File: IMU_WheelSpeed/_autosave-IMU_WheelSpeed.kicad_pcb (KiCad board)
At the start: 2 copper layers, 23 parts, among them J1 Conn_01x06_Socket, J3 Conn_01x03_Socket, U1 PeripheralSOM, U2 LSM6DSL, U4 TPS71518__SC70

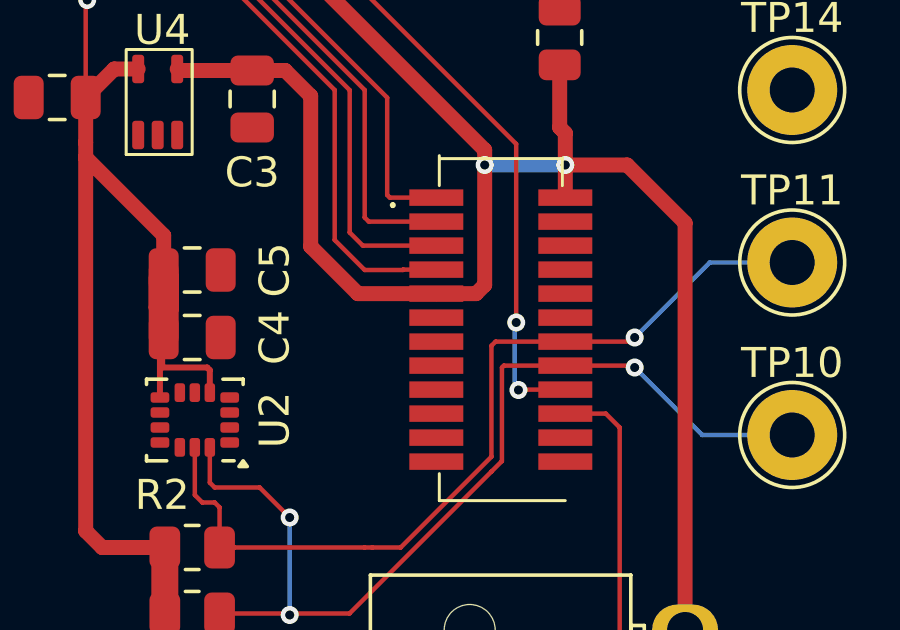
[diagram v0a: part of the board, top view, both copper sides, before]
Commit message: Check up
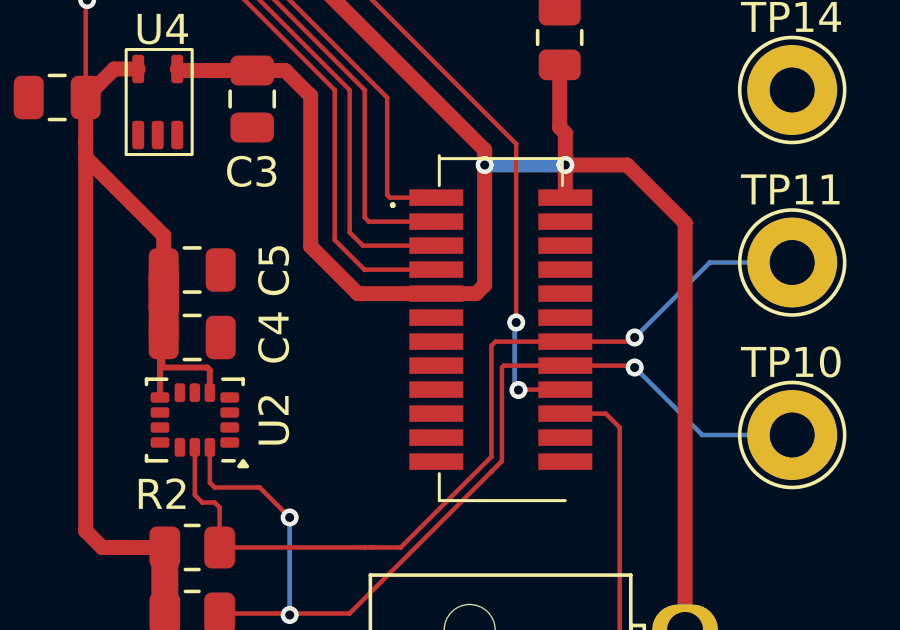
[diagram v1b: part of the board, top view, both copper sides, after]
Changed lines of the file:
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@@
+	)
+	(segment
+		(start 146.25 70.25)
+		(end 145.75 69.75)
+		(width 0.15)
+		(layer "F.Cu")
+		(net 2)
+	)
+	(segment
+		(start 161.13726 84.93726)
+		(end 158.68726 84.93726)
+		(width 0.15)
+		(layer "F.Cu")
+		(net 2)
+	)
+	(segment
+		(start 158.25 79.755025)
+		(end 148.744975 70.25)
+		(width 0.15)
+		(layer "F.Cu")
+		(net 2)
+	)
+	(segment
+		(start 145.75 69.75)
+		(end 145.75 61.93)
+		(width 0.15)
+		(layer "F.Cu")
+		(net 2)
 	)
 	(segment
 		(start 148.744975 70.25)
 		(end 146.25 70.25)
-		(width 0.15)
-		(layer "F.Cu")
-		(net 2)
-	)
-	(segment
-		(start 146.25 70.25)
-		(end 145.75 69.75)
-		(width 0.15)
-		(layer "F.Cu")
-		(net 2)
-	)
-	(segment
-		(start 145.75 69.75)
-		(end 145.75 61.93)
-		(width 0.15)
-		(layer "F.Cu")
-		(net 2)
-	)
-	(segment
-		(start 161.13726 84.93726)
-		(end 158.68726 84.93726)
-		(width 0.15)
-		(layer "F.Cu")
-		(net 2)
-	)
-	(segment
-		(start 158.25 79.755025)
-		(end 148.744975 70.25)
 		(width 0.15)
 		(layer "F.Cu")
@@
 	)
 	(segment
-		(start 163.87476 89.75)
-		(end 163.8875 89.73726)
-		(width 0.15)
-		(layer "F.Cu")
-		(net 5)
-	)
-	(segment
 		(start 163.8 81.55)
 		(end 155.75 73.5)
@@
 	)
 	(segment
+		(start 165.43726 89.73726)
+		(end 163.8875 89.73726)
+		(width 0.15)
+		(layer "F.Cu")
+		(net 5)
+	)
+	(segment
 		(start 163.8875 89.73726)
-		(end 165.43726 89.73726)
+		(end 163.87476 89.75)
 		(width 0.15)
 		(layer "F.Cu")
@@
 	)
 	(segment
+		(start 158.75 79.75)
+		(end 148.25 69.25)
+		(width 0.15)
+		(layer "F.Cu")
+		(net 6)
+	)
+	(segment
+		(start 161.13726 84.13726)
+		(end 158.88726 84.13726)
+		(width 0.15)
+		(layer "F.Cu")
+		(net 6)
+	)
+	(segment
+		(start 158.88726 84.13726)
+		(end 158.75 84)
+		(width 0.15)
+		(layer "F.Cu")
+		(net 6)
+	)
+	(segment
 		(start 158.75 84)
 		(end 158.75 79.75)
@@
 	)
 	(segment
-		(start 158.75 79.75)
-		(end 148.25 69.25)
-		(width 0.15)
-		(layer "F.Cu")
-		(net 6)
-	)
-	(segment
 		(start 148.25 69.25)
 		(end 148.25 61.93)
@@
 	)
 	(segment
-		(start 158.88726 84.13726)
-		(end 158.75 84)
-		(width 0.15)
-		(layer "F.Cu")
-		(net 6)
-	)
-	(segment
-		(start 161.13726 84.13726)
-		(end 158.88726 84.13726)
-		(width 0.15)
-		(layer "F.Cu")
-		(net 6)
-	)
-	(segment
 		(start 130.75 60.75)
 		(end 134.62 60.75)
@@
 	)
 	(segment
+		(start 143.25 70.75)
+		(end 143.25 61.93)
+		(width 0.15)
+		(layer "F.Cu")
+		(net 7)
+	)
+	(segment
+		(start 158.73726 85.73726)
+		(end 157.75 84.75)
+		(width 0.15)
+		(layer "F.Cu")
+		(net 7)
+	)
+	(segment
+		(start 144 71.5)
+		(end 143.25 70.75)
+		(width 0.15)
+		(layer "F.Cu")
+		(net 7)
+	)
+	(segment
 		(start 157.75 84.75)
 		(end 157.75 79.75)
@@
 	)
 	(segment
-		(start 160.03726 85.73726)
-		(end 160.02452 85.75)
-		(width 0.15)
-		(layer "F.Cu")
-		(net 7)
-	)
-	(segment
-		(start 158.75 85.75)
-		(end 157.75 84.75)
-		(width 0.15)
-		(layer "F.Cu")
-		(net 7)
-	)
-	(segment
-		(start 143.25 70.75)
-		(end 143.25 61.93)
-		(width 0.15)
-		(layer "F.Cu")
-		(net 7)
-	)
-	(segment
-		(start 144 71.5)
-		(end 143.25 70.75)
-		(width 0.15)
-		(layer "F.Cu")
-		(net 7)
-	)
-	(segment
 		(start 157.75 79.75)
 		(end 149.5 71.5)
@@
 	(segment
 		(start 161.13726 85.73726)
-		(end 160.03726 85.73726)
-		(width 0.15)
-		(layer "F.Cu")
-		(net 7)
-	)
-	(segment
-		(start 160.02452 85.75)
-		(end 158.75 85.75)
+		(end 158.73726 85.73726)
 		(width 0.15)
 		(layer "F.Cu")
@@
 	)
 	(segment
+		(start 167.25 91)
+		(end 167.25 100.25)
+		(width 0.15)
+		(layer "F.Cu")
+		(net 24)
+	)
+	(segment
+		(start 166.78726 90.53726)
+		(end 167.25 91)
+		(width 0.15)
+		(layer "F.Cu")
+		(net 24)
+	)
+	(segment
+		(start 167.25 100.25)
+		(end 169.43 100.25)
+		(width 0.15)
+		(layer "F.Cu")
+		(net 24)
+	)
+	(segment
 		(start 165.43726 90.53726)
 		(end 166.78726 90.53726)
 		(width 0.15)
 		(layer "F.Cu")
-		(net 24)
-	)
-	(segment
-		(start 167.25 91)
-		(end 167.25 100.25)
-		(width 0.15)
-		(layer "F.Cu")
-		(net 24)
-	)
-	(segment
-		(start 167.25 100.25)
-		(end 169.43 100.25)
-		(width 0.15)
-		(layer "F.Cu")
-		(net 24)
-	)
-	(segment
-		(start 166.78726 90.53726)
-		(end 167.25 91)
-		(width 0.15)
-		(layer "F.Cu")
